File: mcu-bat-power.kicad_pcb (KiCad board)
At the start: 2 copper layers, 41 x 90.9 mm, 35 parts, among them IC1 CN3058E, IC2 HY2112, J1 USB_B_Micro, J2 INDICATORS, J3 PWR, J4 USB, Q1 FS8205, Q2 2N7002, Q3 2N7002, SW1 SW_SPDT, U1 MT3608

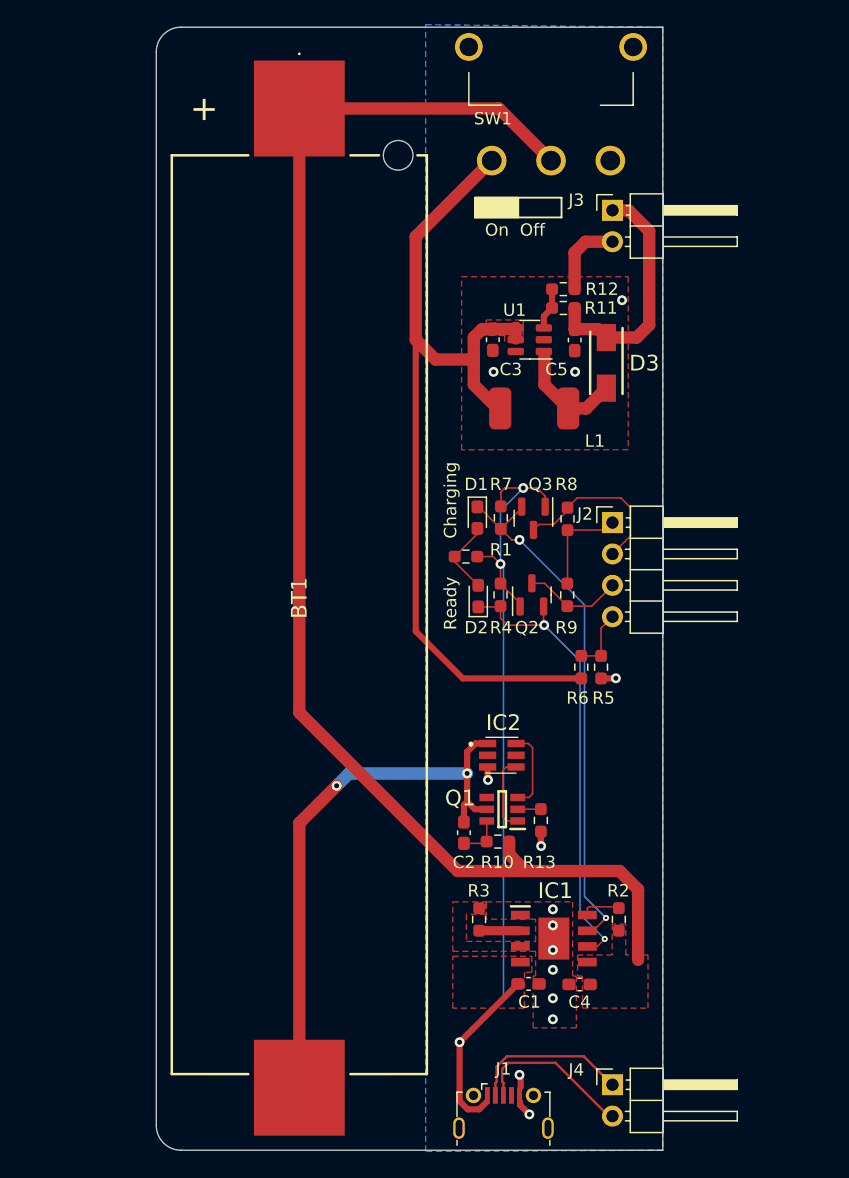
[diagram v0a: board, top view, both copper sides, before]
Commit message: Version 1.0 (sent to fabhouse) + updated readme
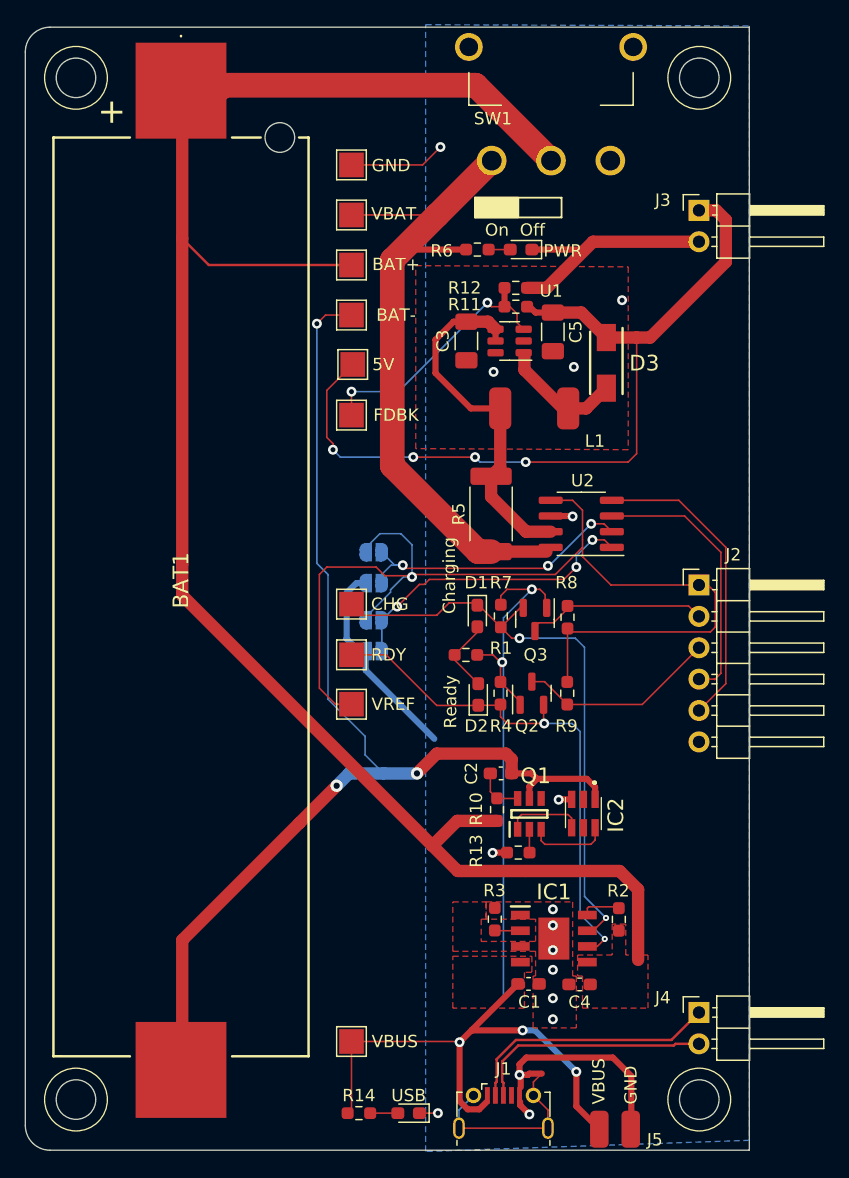
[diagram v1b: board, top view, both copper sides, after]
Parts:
- removed BT1: BH-18650-B1BA002, Chof747 Footprints:BH18650B1BA002
- removed the G*** at (60.6, 74.9)
- added BAT1: BH-18650-B1BA002, Chof747 Footprints:BH18650B1BA002, F.Cu at (51.0, 104.1)
- added D4: PWR, LED_SMD:LED_0603_1608Metric_Pad1.05x0.95mm_HandSolder, F.Cu at (78.5, 77.3)
- added D5: USB, LED_SMD:LED_0603_1608Metric_Pad1.05x0.95mm_HandSolder, F.Cu at (69.4, 147.2)
- added G***: LOGO, Chof747 Logos:LOGO small, B.Cu at (74.2, 104.6)
- added H1: MountingHole, Chof747 Footprints:MountingHole_3.2mm_M3-smallBorder, F.Cu at (42.5, 63.4)
- added H2: MountingHole, Chof747 Footprints:MountingHole_3.2mm_M3-smallBorder, F.Cu at (93.0, 63.4)
- added H3: MountingHole, Chof747 Footprints:MountingHole_3.2mm_M3-smallBorder, F.Cu at (42.5, 146.1)
- added H4: MountingHole, Chof747 Footprints:MountingHole_3.2mm_M3-smallBorder, F.Cu at (93.0, 146.1)
- added J5: PWR, Chof747_Connectors:pad_1x2_1.5mmx3mm, F.Cu at (86.1, 148.5)
- added JP1: A1_H, Jumper:SolderJumper-2_P1.3mm_Open_RoundedPad1.0x1.5mm, B.Cu at (66.6, 107.3)
- added JP2: A1_L, Jumper:SolderJumper-2_P1.3mm_Open_RoundedPad1.0x1.5mm, B.Cu at (66.6, 109.8)
- added JP3: A0_H, Jumper:SolderJumper-2_P1.3mm_Open_RoundedPad1.0x1.5mm, B.Cu at (66.6, 101.8)
- added JP4: A0_L, Jumper:SolderJumper-2_P1.3mm_Open_RoundedPad1.0x1.5mm, B.Cu at (66.6, 104.3)
- added NT1: NetTie_2, NetTie:NetTie-2_SMD_Pad0.5mm, F.Cu at (79.7, 144.0)
- added R14: 1k, Resistor_SMD:R_0603_1608Metric_Pad0.98x0.95mm_HandSolder, F.Cu at (65.4, 147.2)
- added TP1: GND, TestPoint:TestPoint_Pad_2.0x2.0mm, F.Cu at (64.8, 70.5)
- added TP10: CHG, TestPoint:TestPoint_Pad_2.0x2.0mm, F.Cu at (64.8, 106.0)
- added TP2: VBAT, TestPoint:TestPoint_Pad_2.0x2.0mm, F.Cu at (64.8, 74.5)
- added TP3: BAT+, TestPoint:TestPoint_Pad_2.0x2.0mm, F.Cu at (64.8, 78.5)
- added TP4: BAT-, TestPoint:TestPoint_Pad_2.0x2.0mm, F.Cu at (64.8, 82.6)
- added TP5: 5V, TestPoint:TestPoint_Pad_2.0x2.0mm, F.Cu at (64.9, 86.6)
- added TP6: FDBK, TestPoint:TestPoint_Pad_2.0x2.0mm, F.Cu at (64.8, 90.7)
- added TP7: VBUS, TestPoint:TestPoint_Pad_2.0x2.0mm, F.Cu at (64.8, 141.4)
- added TP8: VREF, TestPoint:TestPoint_Pad_2.0x2.0mm, F.Cu at (64.8, 114.1)
- added TP9: RDY, TestPoint:TestPoint_Pad_2.0x2.0mm, F.Cu at (64.8, 110.1)
- added U2: INA219AxD, Package_SO:SOIC-8_3.9x4.9mm_P1.27mm, F.Cu at (83.4, 99.5)
- C3, C5: footprint Capacitor_SMD:C_0603_1608Metric_Pad1.08x0.95mm_HandSolder -> Capacitor_SMD:C_1206_3216Metric_Pad1.33x1.80mm_HandSolder
- J2: footprint Connector_PinHeader_2.54mm:PinHeader_1x04_P2.54mm_Horizontal -> Connector_PinHeader_2.54mm:PinHeader_1x06_P2.54mm_Horizontal
- R5: value 470k -> 0R1; footprint Resistor_SMD:R_0603_1608Metric_Pad0.98x0.95mm_HandSolder -> Resistor_SMD:R_2512_6332Metric_Pad1.40x3.35mm_HandSolder
- R6: value 470k -> 1k
- moved R6 35.3 mm to (75.0, 77.3), turned to 0 degrees
- moved R5 14.4 mm to (76.1, 98.7), turned to 90 degrees
- moved J4 9.12 mm to (92.9, 139.1)
- moved J2 8.63 mm to (92.9, 104.5)
- moved Q1 8.31 mm to (83.6, 122.3), turned to -90 degrees
- moved Q3 8.19 mm to (79.7, 107.2)
- moved D2 7.96 mm to (75.1, 113.3)
- moved R8 7.96 mm to (82.3, 107.1)
- moved D1 7.96 mm to (75.0, 107.0)
- moved Q2 7.96 mm to (79.4, 113.2)
- moved R1 7.96 mm to (74.1, 110.1)
- moved R4 7.96 mm to (76.9, 113.2)
- moved R7 7.96 mm to (76.9, 107.0)
- moved R9 7.96 mm to (82.3, 113.2)
- moved J3 7.00 mm to (92.9, 74.1)
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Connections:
- net Net-(U1-FB) renamed FDBK
- C3 pad 1: VBAT -> VBAT_M
- J1 pad 6: unconnected-(J1-Shield-Pad6) -> Net-(J1-Shield)
- J2 pad 4: /BAT_SENSE -> SDA
- L1 pad 1: VBAT -> VBAT_M
- R5 pad 1: /BAT_SENSE -> VBAT
- R5 pad 2: VBAT -> VBAT_M
- R6 pad 1: GND -> VBAT
- R6 pad 2: /BAT_SENSE -> Net-(D4-A)
- U1 pad 4: VBAT -> VBAT_M
- U1 pad 5: VBAT -> VBAT_M
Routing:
- net VREF: track 8.23 -> 86.5 mm, vias 0 -> 1
- net GND: track 12.2 -> 69.5 mm, vias 14 -> 16
- net BAT-: track 46.2 -> 98.0 mm, vias 2 -> 3
- net +5V: track 19.5 -> 68.1 mm, vias 0 -> 4
- net BAT+: track 113.0 -> 146.7 mm
- net VBAT_M: track 0.00 -> 29.2 mm
- net SCL: track 0.00 -> 24.9 mm
- net Net-(JP1-A): track 0.00 -> 24.2 mm, vias 0 -> 3
- net Net-(JP3-A): track 0.00 -> 23.6 mm, vias 0 -> 3
- net SDA: track 0.00 -> 21.8 mm
- net VBUS: track 73.6 -> 95.0 mm, vias 3 -> 5
- net FDBK: track 3.41 -> 21.3 mm, vias 0 -> 2
- net Net-(J1-Shield): track 0.00 -> 15.5 mm
- net VBAT: track 72.4 -> 57.1 mm
- net Net-(J2-Pin_3): track 8.00 -> 16.2 mm
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- removed copper zone on F.Cu, net VBAT
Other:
- board size 41 x 90.9 mm -> 58.6 x 90.9 mm
- board text added: "Battery Power (LiFePo4) v1.0 (2024)"
- board text added: "INA219 Adr."
- board text added: "SCL(I2C)"
- board text added: "SDA(I2C)"
- board text added: "VBUS"
- board text added: "VREF"
- board text removed: "BAT V Sense (VBAT / 2)"
- board text removed: "Battery Power Board (LiFePo4) v1.0 (2023)"
- board text removed: "VREF (=MCU Voltage)"
